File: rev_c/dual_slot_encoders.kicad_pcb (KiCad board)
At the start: 2 copper layers, 50 x 25 mm, 15 parts, among them U1 GP1S094HCZ0F, U2 GP1S094HCZ0F, U3 GPS1S97HCZ0F, U4 GPS1S97HCZ0F

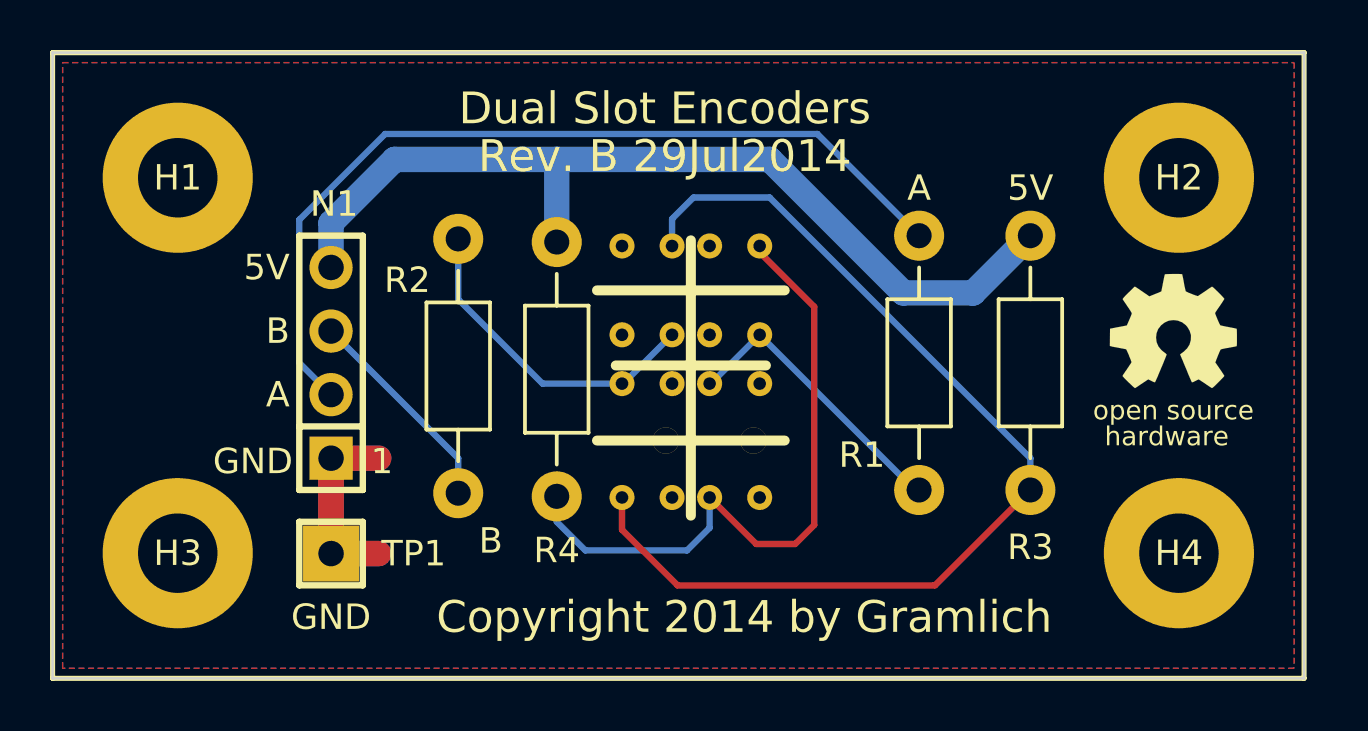
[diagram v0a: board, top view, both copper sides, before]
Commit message: Rev. C is pretty much done.
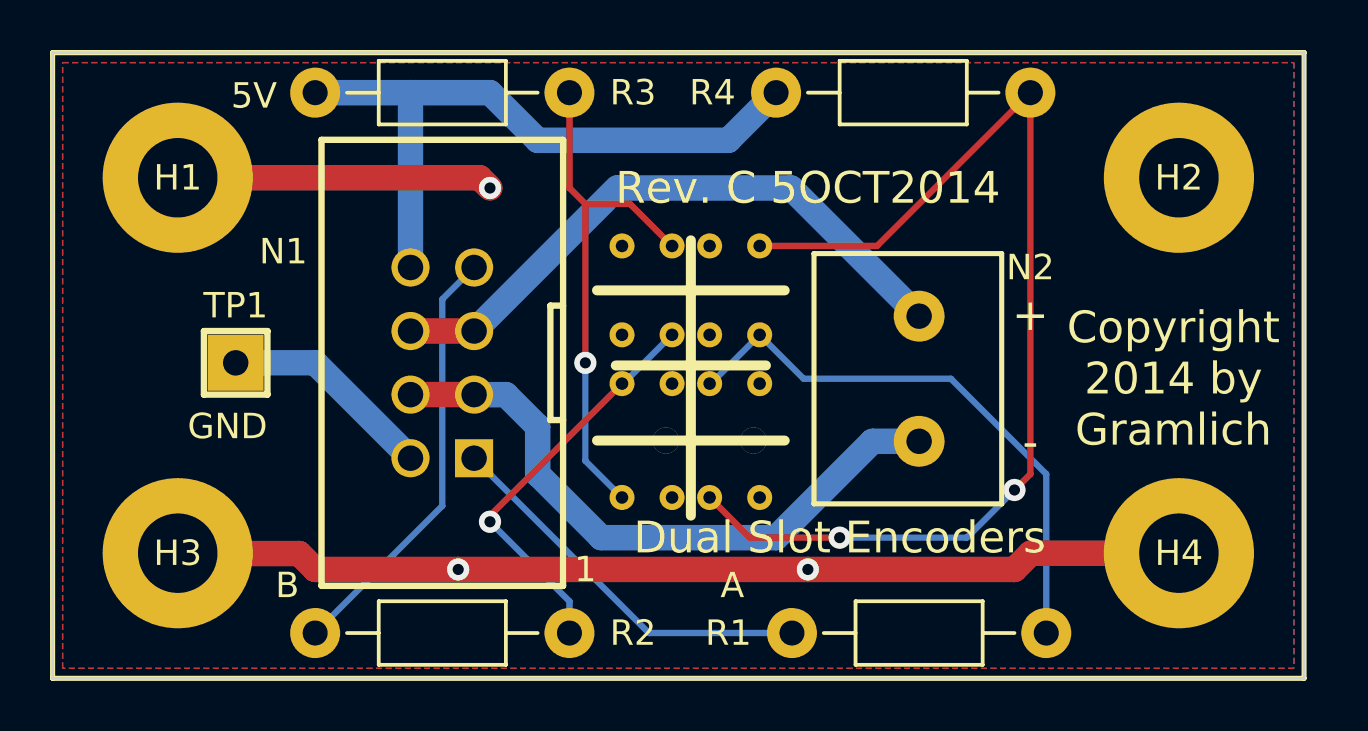
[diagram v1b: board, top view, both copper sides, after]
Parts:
- removed Z1: OSHW_LOGO, Dual_Slot_Encoders_Rev_B:OSHW_LOGO_200mil
- added G1: OSHW_LOGO, dual_slot_encoders:OSHW_LOGO_200mil, B.Cu at (142.2, 110.5)
- added N2: MOTOR_CONN, dual_slot_encoders:5MM_TERMINAL_BLOCK_2_POS, F.Cu at (134.6, 113.0)
- H1, H2, H3, H4: footprint Dual_Slot_Encoders_Rev_B:MountingHole_3mm -> dual_slot_encoders:MountingHole_3mm
- N1: value ENCODER_CONNECTOR -> MOTOR_ENCODER_CONN; footprint Dual_Slot_Encoders_Rev_B:Pin_Header_Straight_1x04 -> dual_slot_encoders:Pin_Header_Straight_2x04_Shrouded
- R1, R2, R3, R4: footprint Dual_Slot_Encoders_Rev_B:Resistor_Horizontal_400 -> dual_slot_encoders:Resistor_Horizontal_400
- TP1: footprint Dual_Slot_Encoders_Rev_B:Pin_Header_Straight_1x01 -> dual_slot_encoders:Pin_Header_Straight_1x01
- U1, U2: footprint Dual_Slot_Encoders_Rev_B:GP1S094HCZ0F -> dual_slot_encoders:GP1S094HCZ0F
- U3, U4: footprint Dual_Slot_Encoders_Rev_B:GP1S097HCZ0F -> dual_slot_encoders:GP1S097HCZ0F
- moved R3 25.9 mm to (115.6, 101.6), turned to 180 degrees
- moved R4 17.7 mm to (134.0, 101.6), turned to 180 degrees
- moved R1 10.8 mm to (134.6, 123.2), turned to 180 degrees
- moved R2 10.7 mm to (115.6, 123.2), turned to 180 degrees
- moved TP1 8.52 mm to (107.3, 112.4)
- moved N1 4.44 mm to (115.6, 112.4)
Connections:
- N1 pad 1: /GND -> /A
- N1 pad 2: /A -> /GND
- N1 pad 3: /B -> /MOTOR-
- N1 pad 4: /5V -> /MOTOR-
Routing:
- net /GND: track 15.2 -> 61.7 mm, vias 0 -> 3
- net /MOTOR-: track 0.00 -> 25.4 mm
- net /MOTOR+: track 0.00 -> 24.8 mm
- net Net-(R3-Pad1): track 41.4 -> 21.2 mm, vias 0 -> 1
- net /A: track 35.4 -> 15.6 mm
- net Net-(R4-Pad1): track 26.6 -> 43.1 mm, vias 0 -> 2
- net Net-(R1-Pad1): track 11.7 -> 22.9 mm
- net /5V: track 37.2 -> 27.0 mm
- net /B: track 8.58 -> 17.2 mm
- net Net-(R2-Pad1): track 13.2 -> 16.3 mm, vias 0 -> 1
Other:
- board text added: "+"
- board text added: "-"
- board text added: "Rev. C 5OCT2014"
- board text removed: "Rev. B 29Jul2014"
